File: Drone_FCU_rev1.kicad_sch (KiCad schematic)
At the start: 31 parts, among them J1 Conn_01x02_Pin, P1 USB_C_Plug_USB2.0, SW1 SW_Push, U1 STM32F722VETx, Y2 16MHz

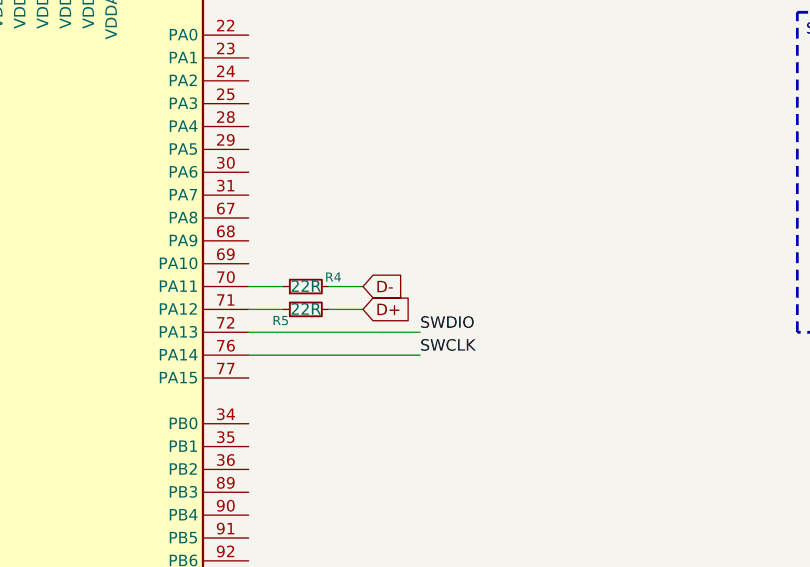
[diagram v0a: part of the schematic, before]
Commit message: Updates
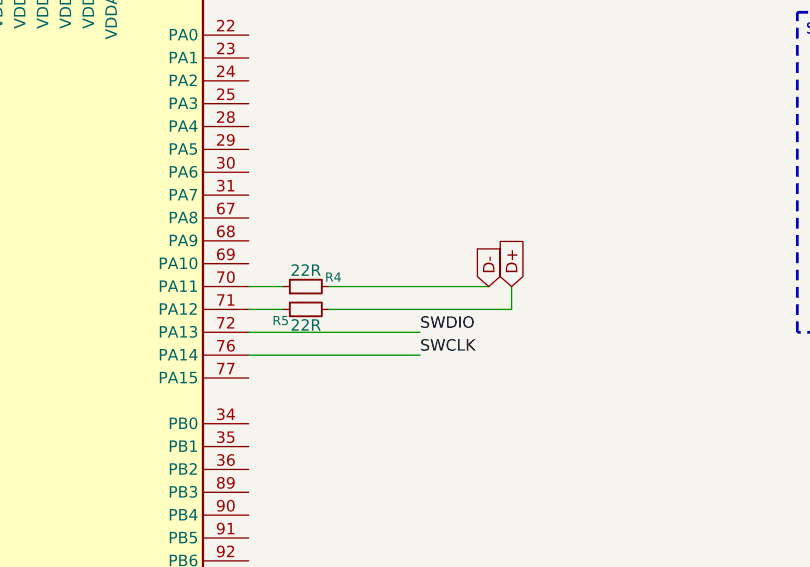
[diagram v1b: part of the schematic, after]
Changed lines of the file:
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@@
 	(wire
 		(pts
-			(xy 241.3 107.95) (xy 245.11 107.95)
-		)
-		(stroke
-			(width 0)
-			(type default)
-		)
-	)
-	(wire
-		(pts
 			(xy 232.41 113.03) (xy 251.46 113.03)
 		)
@@
 	(wire
 		(pts
-			(xy 241.3 105.41) (xy 245.11 105.41)
+			(xy 241.3 105.41) (xy 259.08 105.41)
 		)
 		(stroke
@@
 	(wire
 		(pts
+			(xy 261.62 105.41) (xy 261.62 107.95)
+		)
+		(stroke
+			(width 0)
+			(type default)
+		)
+	)
+	(wire
+		(pts
 			(xy 353.06 49.53) (xy 368.3 49.53)
 		)
@@
 	(wire
 		(pts
+			(xy 261.62 107.95) (xy 241.3 107.95)
+		)
+		(stroke
+			(width 0)
+			(type default)
+		)
+	)
+	(wire
+		(pts
 			(xy 209.55 212.09) (xy 209.55 213.36)
 		)
@@
 	(global_label "D+"
 		(shape input)
-		(at 245.11 107.95 0)
+		(at 261.62 105.41 90)
 		(fields_autoplaced yes)
 		(effects
@@
 		)
 		(property "Intersheetrefs" "${INTERSHEET_REFS}"
-			(at 250.9376 107.95 0)
+			(at 261.62 99.5824 90)
 			(effects
 				(font
@@
 	(global_label "D-"
 		(shape input)
-		(at 245.11 105.41 0)
+		(at 259.08 105.41 90)
 		(fields_autoplaced yes)
 		(effects
@@
 		)
 		(property "Intersheetrefs" "${INTERSHEET_REFS}"
-			(at 250.9376 105.41 0)
+			(at 259.08 99.5824 90)
 			(effects
 				(font
@@
 		)
 		(property "Value" "22R"
-			(at 238.76 107.95 90)
+			(at 238.76 109.728 90)
 			(effects
 				(font
@@
 		)
 		(property "Value" "22R"
-			(at 238.76 105.41 90)
+			(at 238.76 103.632 90)
 			(effects
 				(font
